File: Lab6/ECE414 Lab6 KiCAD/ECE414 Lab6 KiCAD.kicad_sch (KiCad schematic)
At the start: 9 parts, among them M1 Motor_DC, Q1 IRLB8721PBF, SW1 SW_Push, U1 Pico, U2 2478, U3 4N35

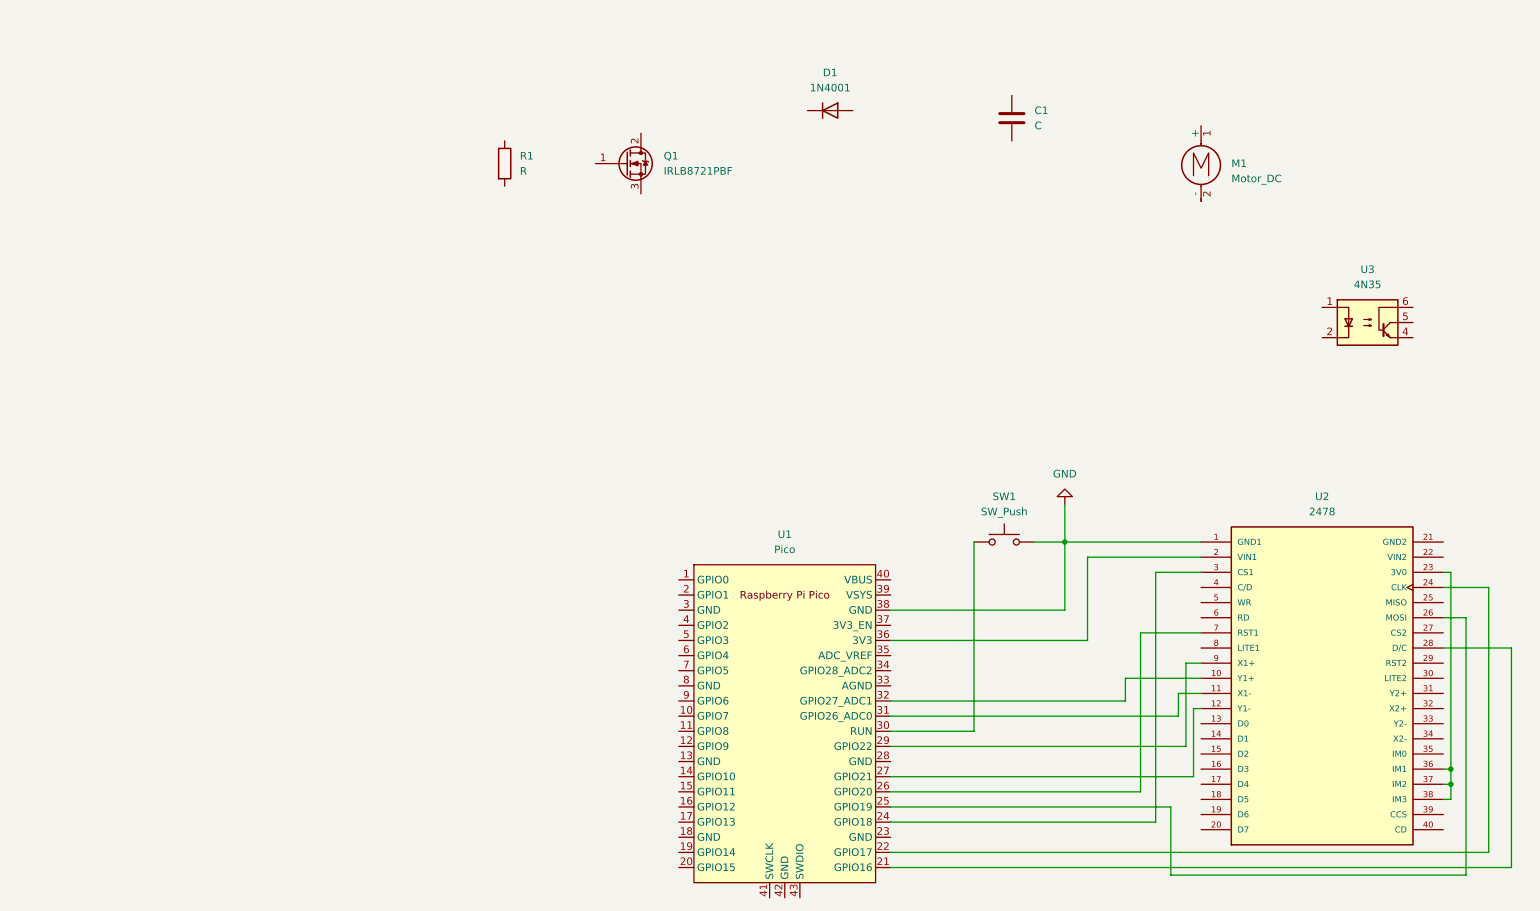
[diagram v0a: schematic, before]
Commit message: kicad a little better
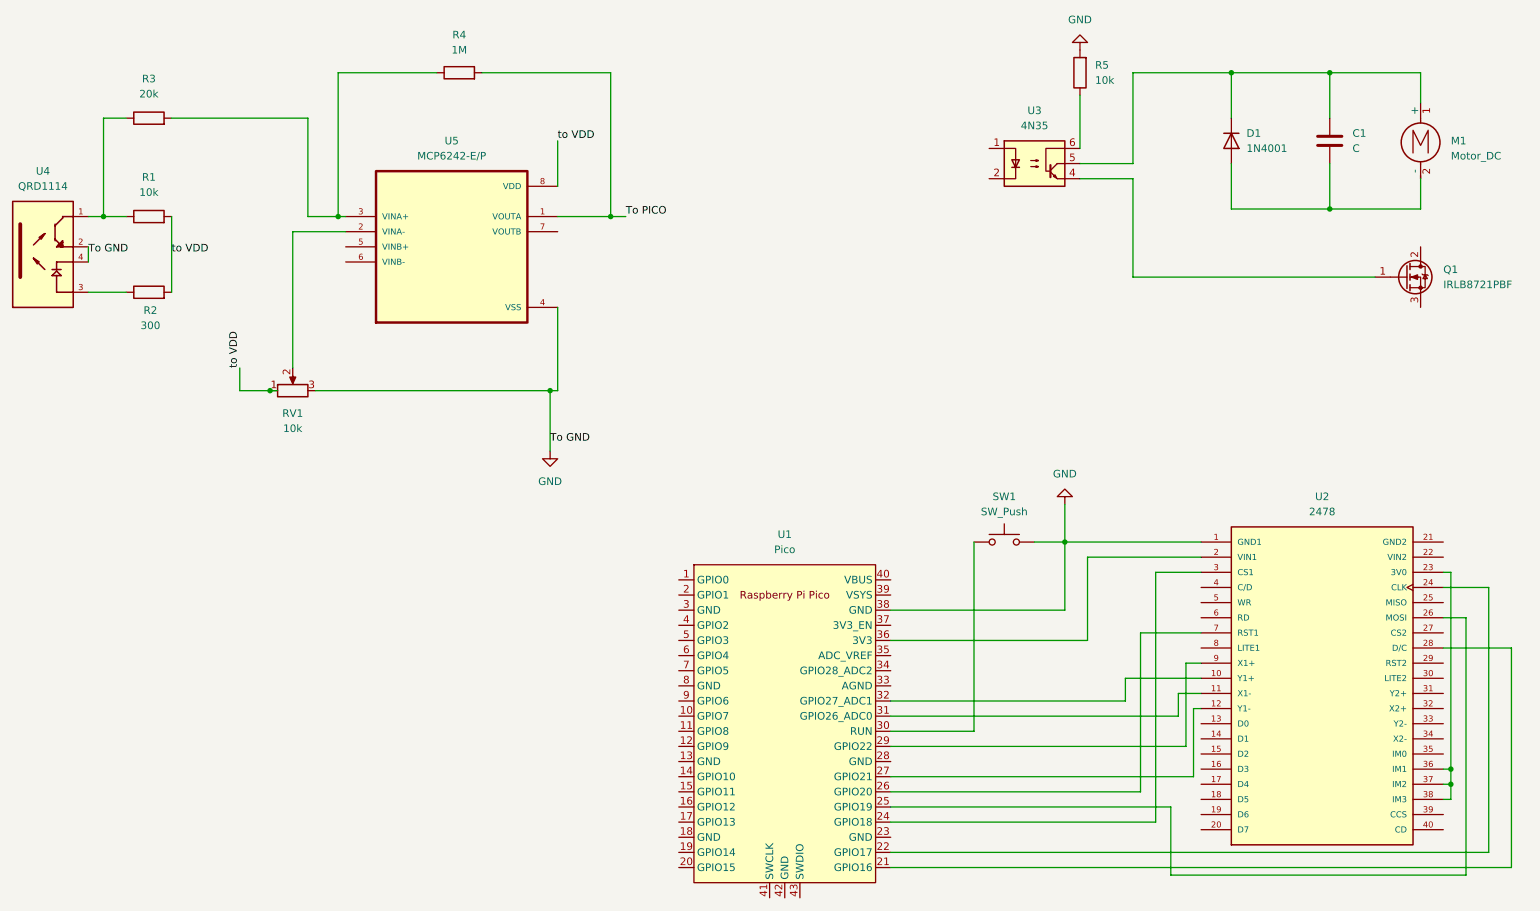
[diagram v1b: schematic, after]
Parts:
- added R2: 300, symbol Device:R
- added R3: 20k, symbol Device:R
- added R4: 1M, symbol Device:R
- added R5: 10k, symbol Device:R
- added RV1: 10k, symbol Device:R_Potentiometer
- added U4: QRD1114, ONS_QRD1114, symbol QRD1114:QRD1114
- added U5: MCP6242-E/P, DIP787W46P254L927H533Q8, symbol MCP6242-E_P:MCP6242-E/P
- R1: value R -> 10k
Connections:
- net GND: now also R5.2, RV1.3, U4.2, U4.4, U5.4 (VSS)
- net at Q1.1 (G): now also U3.4
- net at M1.1 (+): now also C1.2, D1.1 (K), U3.5
- net at M1.2 (-): now also C1.1, D1.2 (A)
- net at R1.1: now also R3.1, U4.1
- net to VDD: now reaches R1.2
- net to VDD: now also R2.2, RV1.1, U5.8 (VDD)
- net at U3.6: now also R5.1
- new net: RV1.2, U5.2 (VINA-)
- new net: R3.2, R4.1, U5.3 (VINA+)
- new net: R2.1, U4.3
- new net To PICO: R4.2, U5.1 (VOUTA)
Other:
- moved on the sheet: C1, D1, M1, Q1, R1, U3
